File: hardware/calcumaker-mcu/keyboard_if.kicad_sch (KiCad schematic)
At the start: 2 parts, among them J5 TO KEYBOARD (stack), J6 TO KEYBOARD (FFC)

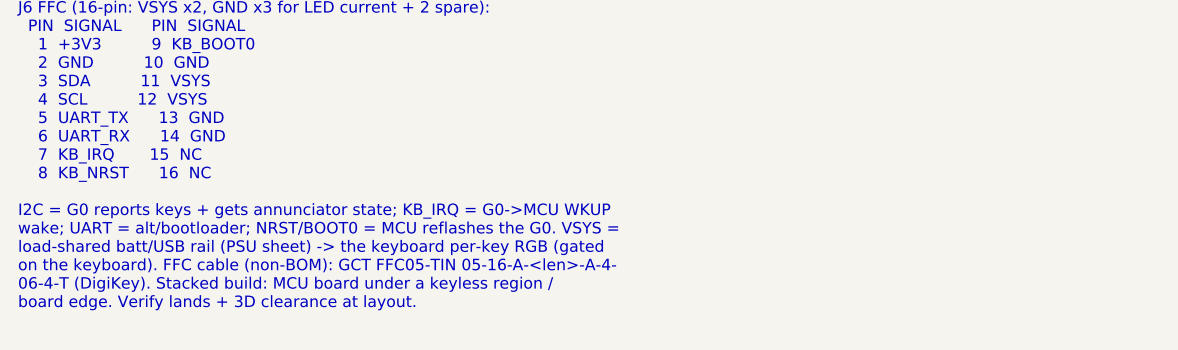
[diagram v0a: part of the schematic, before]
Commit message: Checkpoint
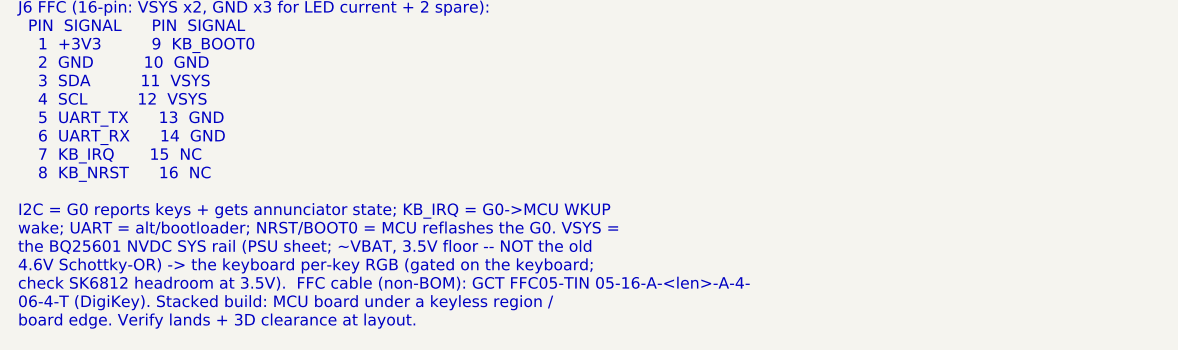
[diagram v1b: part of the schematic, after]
